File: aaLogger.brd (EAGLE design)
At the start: 88.9 x 48.3 mm, 55 parts, among them Q1 IRLML6244TR, U1 MCP1640C, U2 ATmega328P-AU

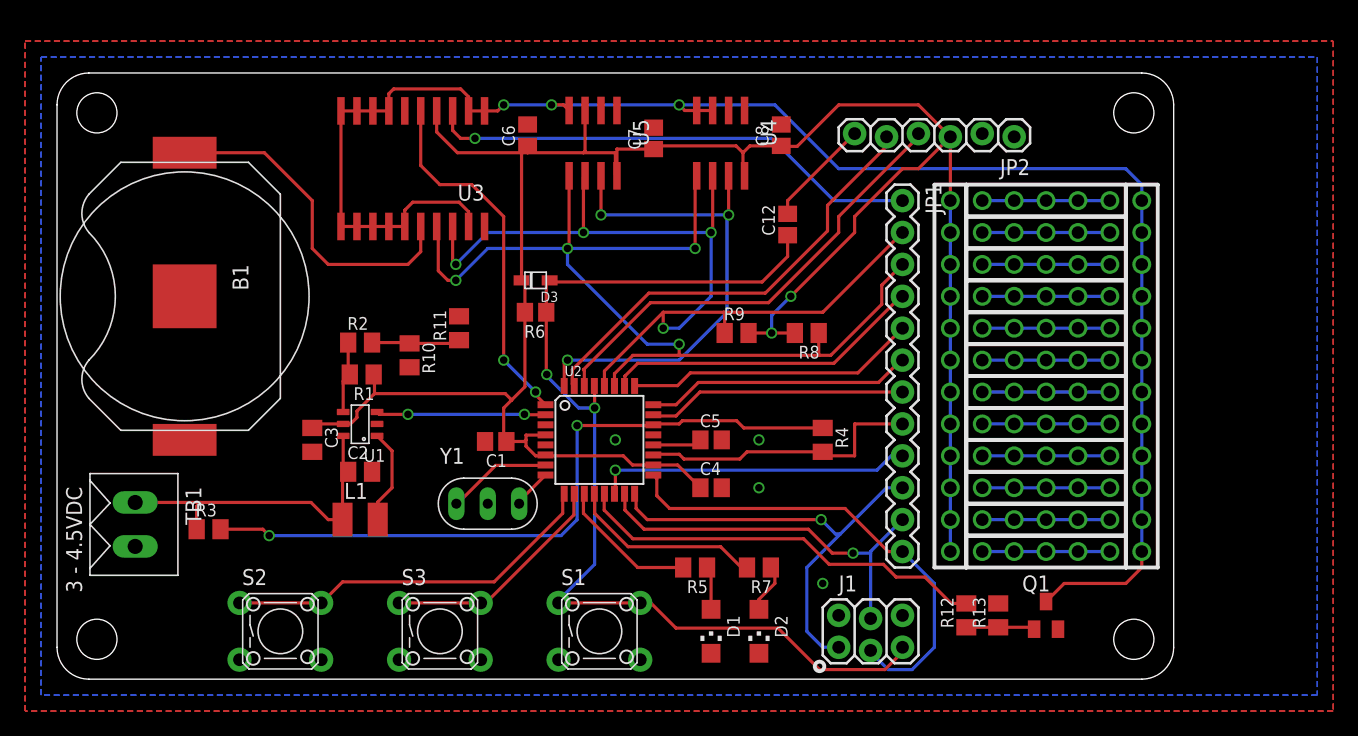
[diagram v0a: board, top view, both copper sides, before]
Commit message: Near final.
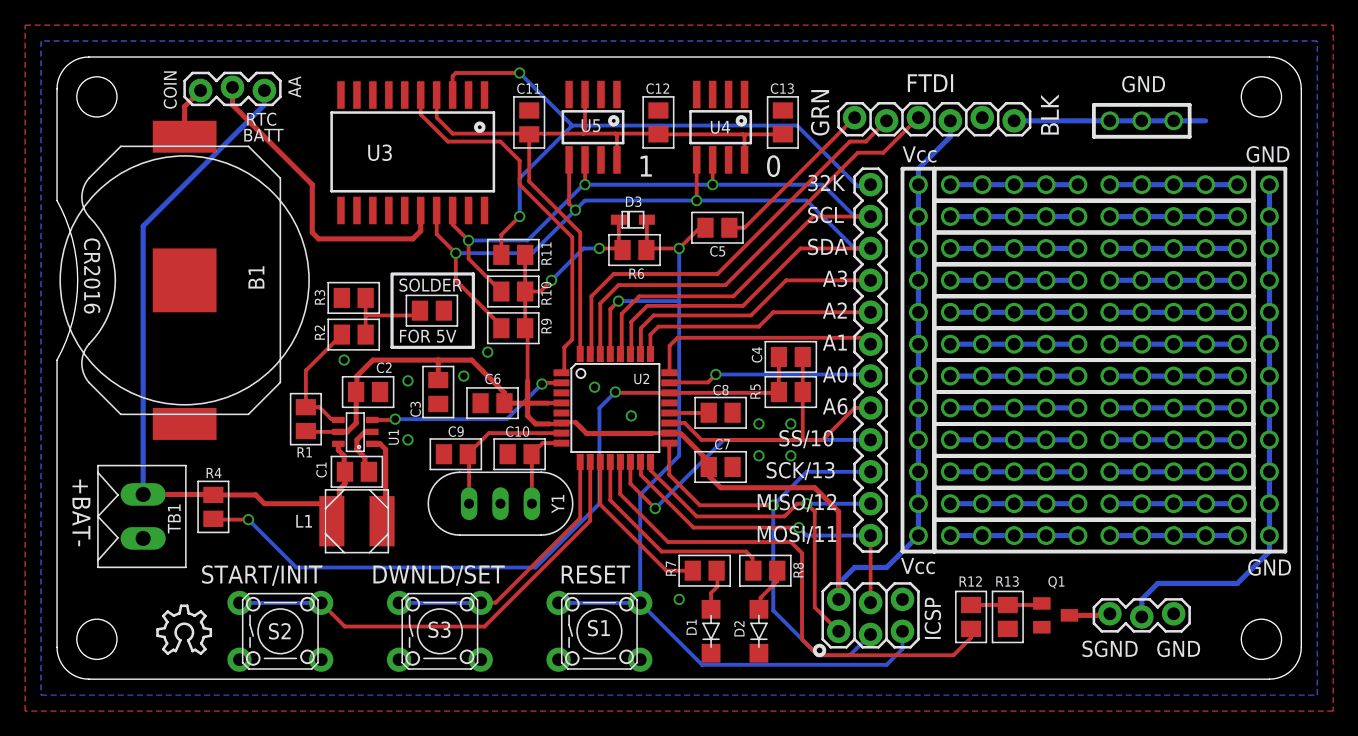
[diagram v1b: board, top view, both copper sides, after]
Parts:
- added C10, C9: 27pF, _jc:M0805
- added C11, C13: 100nF, _jc:M0805
- added JMP1: solder jumper, _jc:M0805
- added JP3: GNDSEL, SparkFun:1X03_LOCK
- added JP4: RTC BACKUP, SparkFun:1X03_LOCK
- added LOGO1, LOGO2: OSHW_LOGO_8MILX0150-NT, ohw-logo:OSHW_8X150_NOTEXT
- added PR13: (no value), _jc:PROTO-3
- B1: value (none) -> CR2016
- C1: value 100nF -> 10uF; device _jc:C0805 -> _jc:M0805
- C12, C4, C5, C6, C7, C8: device _jc:C0805 -> _jc:M0805
- J1: value (none) -> ICSP
- L1: device _jc:R1210 -> _jc:NRS5020
- PR1, PR10, PR11, PR12, PR2, PR3, PR4, PR5, PR6, PR7, PR8, PR9: value PROTO-5 -> PROTO-10; device _jc:PROTO-5 -> _jc:PROTO-10
- R10: value 249K -> 2.2K
- R11: value solder jumper -> 10K
- R12: value 100 -> 220
- R3: value 47.5K -> 249K
- R4: value 10K -> 47.5K
- R5: value 2.2K -> 10K
- R6: device _jc:R0805 -> _jc:M0805
- S1: value (none) -> RESET
- S2: value (none) -> START/INIT
- S3: value (none) -> DL/SET
- TB1: value 3 - 4.5VDC -> +BAT-
- U3: value (none) -> DS3232
- U4, U5: value (none) -> M24M02
- Y1: value (none) -> 8MHz; device _jc:ZTT-RESONATOR -> _jc:RESONATOR
- moved R4 48.8 mm to (12.4, 13.7)
- moved C7 26.7 mm to (52.8, 16.9), turned to 0 degrees
- moved C8 22.6 mm to (52.8, 21.2), turned to 0 degrees
- moved R3 21.7 mm to (23.6, 30.4), turned to 180 degrees
- moved C6 21.5 mm to (34.7, 22.0), turned to 180 degrees
- moved R8 19.2 mm to (56.4, 8.64)
- moved R9 17.8 mm to (36.3, 27.9)
- moved C5 16.9 mm to (52.6, 35.9)
- moved R5 15.9 mm to (58.4, 22.9), turned to 0 degrees
- moved PR1 14.5 mm to (82.5, 39.4), turned to 0 degrees
- moved C12 13.1 mm to (47.9, 44.3)
- moved C4 12.2 mm to (58.4, 25.7)
- moved C1 11.3 mm to (23.9, 16.5), turned to 0 degrees
- moved C3 10.7 mm to (30.4, 22.9)
- moved U$2 10.2 mm to (96.5, 25.4)
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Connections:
- removed net /WC: U2.32, U4.7, U5.7
- removed net PGND: Q1.3, U$2.PAD01, U$2.PAD02, U$2.PAD03, U$2.PAD04, U$2.PAD05, U$2.PAD06, U$2.PAD07, U$2.PAD08, U$2.PAD09, U$2.PAD10, U$2.PAD11, U$2.PAD12, U3.1, U3.10, U3.11, U3.12, U3.13, U3.14, U3.15, U3.19, U3.2, U3.7, U3.8, U3.9, U4.3, U4.4, U5.4
- new net N$10: PR3.10, PR3.6, PR3.7, PR3.8, PR3.9
- new net N$14: PR4.10, PR4.6, PR4.7, PR4.8, PR4.9
- new net N$15: PR6.10, PR6.6, PR6.7, PR6.8, PR6.9
- new net N$28: PR7.10, PR7.6, PR7.7, PR7.8, PR7.9
- new net N$30: PR8.10, PR8.6, PR8.7, PR8.8, PR8.9
- new net N$31: PR9.10, PR9.6, PR9.7, PR9.8, PR9.9
- new net N$32: PR10.10, PR10.6, PR10.7, PR10.8, PR10.9
- new net N$33: PR11.10, PR11.6, PR11.7, PR11.8, PR11.9
- new net N$34: PR12.10, PR12.6, PR12.7, PR12.8, PR12.9
- new net N$35: JP4.2, U3.16
- new net N$36: JP3.1, Q1.3
- new net N$4: PR1.10, PR1.6, PR1.7, PR1.8, PR1.9
- new net N$5: PR5.10, PR5.6, PR5.7, PR5.8, PR5.9
- new net N$9: PR2.10, PR2.6, PR2.7, PR2.8, PR2.9
- new net SGND: JP3.2, U$2.1, U$2.10, U$2.11, U$2.12, U$2.2, U$2.3, U$2.4, U$2.5, U$2.6, U$2.7, U$2.8, U$2.9
- new net SPWR: R12.2, U2.13
- net /RESET: now also C5.1; no longer C12.1
- net 32KHZ: now also R11.1
- net ADC6: now also C4.2, R5.2; no longer R4.2
- net ADC7: now also C4.1, R4.2, R5.1; no longer R3.2, R4.1
- net BAT: now also C1.1, JP4.1, L1.P$1, R4.1; no longer C2.1, L1.1, R3.1
- net GND: now also C10.2, C11.2, C12.2, C13.2, C9.2, JMP1.2, JP3.3, PR13.1, PR13.2, PR13.3, R3.2, U3.1, U3.10, U3.11, U3.12, U3.13, U3.14, U3.15, U3.19, U3.2, U3.7, U3.8, U3.9, U4.3, U4.4, U4.7, U5.4, U5.7; no longer C4.2, C5.2, R10.2, R11.2
- net LED1: now also R7.2; no longer R5.2
- net LED2: now also R8.2; no longer R7.2
- net MISO: now also JP1.11; no longer JP1.10
- net MOSI: now also JP1.12; no longer JP1.11
- net N$1: now also JP4.3; no longer U3.16
- net N$11: now also C10.1
- net N$12: now also JMP1.1, R3.1; no longer R10.1, R11.1
- net N$13: now also C8.1; no longer C5.1
- net N$2: now also R7.1; no longer R5.1
- net N$3: now also R8.1; no longer R7.1
- net N$7: now also L1.P$2; no longer L1.2
- net N$8: now also C9.1
- net PPWR: now also C11.1, C12.1, C13.1, U2.32, U3.4, U4.8, U5.3, U5.8; no longer R12.2, U2.13
- net RST: now also C5.2; no longer C12.2
- net SCK: now also JP1.10; no longer JP1.12
- net SCL: now also R10.1; no longer R9.1
- net SDA: now also R9.1; no longer R8.1
- net SW2: now also U2.10; no longer U2.9
- net SW3: now also U2.9; no longer U2.10
- net VCC: now also C2.1, R10.2, R11.2, U$1.1, U$1.10, U$1.11, U$1.12, U$1.2, U$1.3, U$1.4, U$1.5, U$1.6, U$1.7, U$1.8, U$1.9; no longer C1.1, C4.1, C8.1, R8.2, U$1.PAD01, U$1.PAD02, U$1.PAD03, U$1.PAD04, U$1.PAD05, U$1.PAD06, U$1.PAD07, U$1.PAD08, U$1.PAD09, U$1.PAD10, U$1.PAD11, U$1.PAD12, U3.4, U4.8, U5.3, U5.8
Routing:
- net PGND: track 135.6 -> 0.00 mm, vias 3 -> 0
- net VCC: track 177.4 -> 132.2 mm
- net SGND: track 0.00 -> 42.3 mm
- net SPWR: track 0.00 -> 41.1 mm
- net /WC: track 40.6 -> 0.00 mm, vias 3 -> 0
- net BAT: track 26.4 -> 59.5 mm
- net N$35: track 0.00 -> 24.9 mm
- net PPWR: track 33.2 -> 56.5 mm
- net N$1: track 27.1 -> 4.21 mm
- net GND: track 0.00 -> 19.7 mm, vias 4 -> 12
- net 32KHZ: track 39.7 -> 51.3 mm, vias 1 -> 2
- net N$9: track 0.00 -> 10.2 mm
- net N$5: track 0.00 -> 10.2 mm
- net N$4: track 0.00 -> 10.2 mm
- net N$34: track 0.00 -> 10.2 mm
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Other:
- board size 88.9 x 48.3 mm -> 99.1 x 49.5 mm
- board text added: "0"
- board text added: "1"
- board text added: "32K"
- board text added: "A0"
- board text added: "A1"
- board text added: "A2"
- board text added: "A3"
- board text added: "A6"
- board text added: "AA"
- board text added: "BATT"
- board text added: "BLK"
- board text added: "CC BY-SA jc 0213 v1"
- board text added: "COIN"
- board text added: "DWNLD/SET"
- board text added: "Double-A Datalogger"
- board text added: "FOR 5V"
- board text added: "FTDI"
- board text added: "GND"
- board text added: "GRN"
- board text added: "ICSP"
- board text added: "MISO/12"
- board text added: "MOSI/11"
- board text added: "RESET"
- board text added: "RTC"
- board text added: "SCK/13"
- board text added: "SCL"
- board text added: "SDA"
- board text added: "SGND"
- board text added: "SOLDER"
- board text added: "SS/10"
- board text added: "START/INIT"
- board text added: "Vcc"
- board text added: "open source"
